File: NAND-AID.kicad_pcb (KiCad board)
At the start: 2 copper layers, 33.7 x 21.4 mm, 20 parts

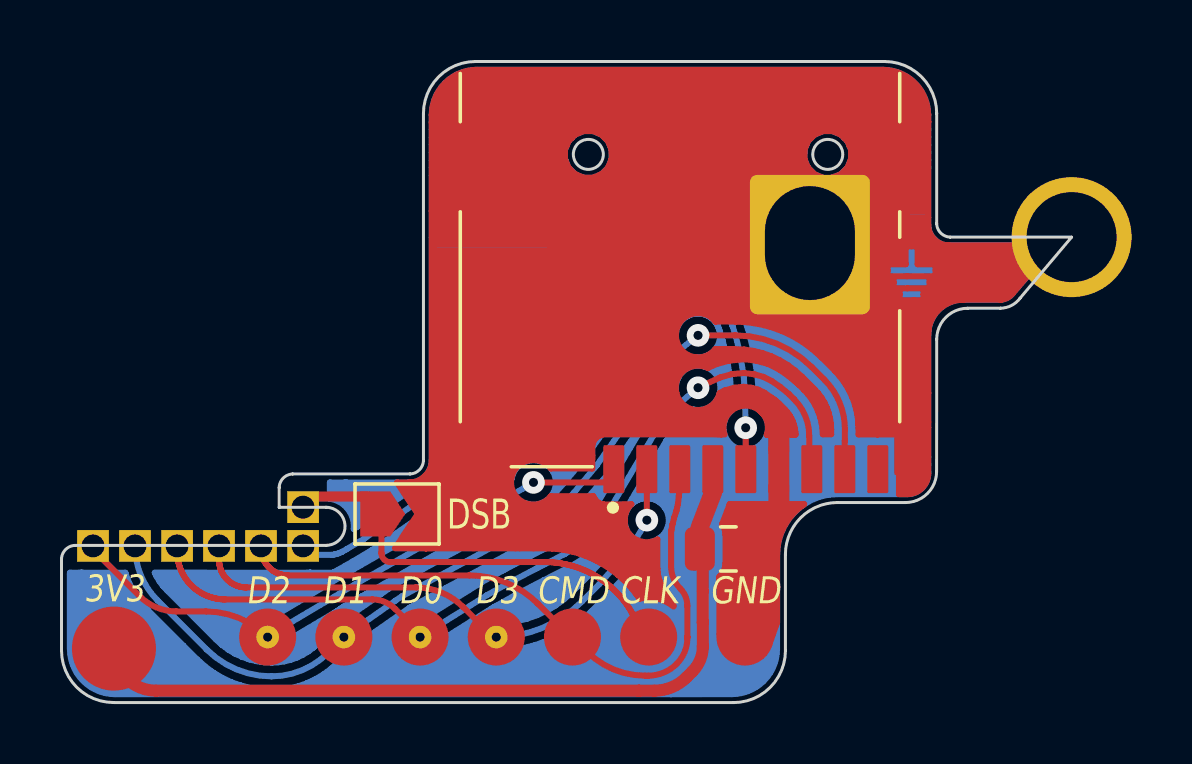
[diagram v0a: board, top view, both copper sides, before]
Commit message: Add logo
Signed-off-by: Thomas Rohloff <v10lator@myway.de>
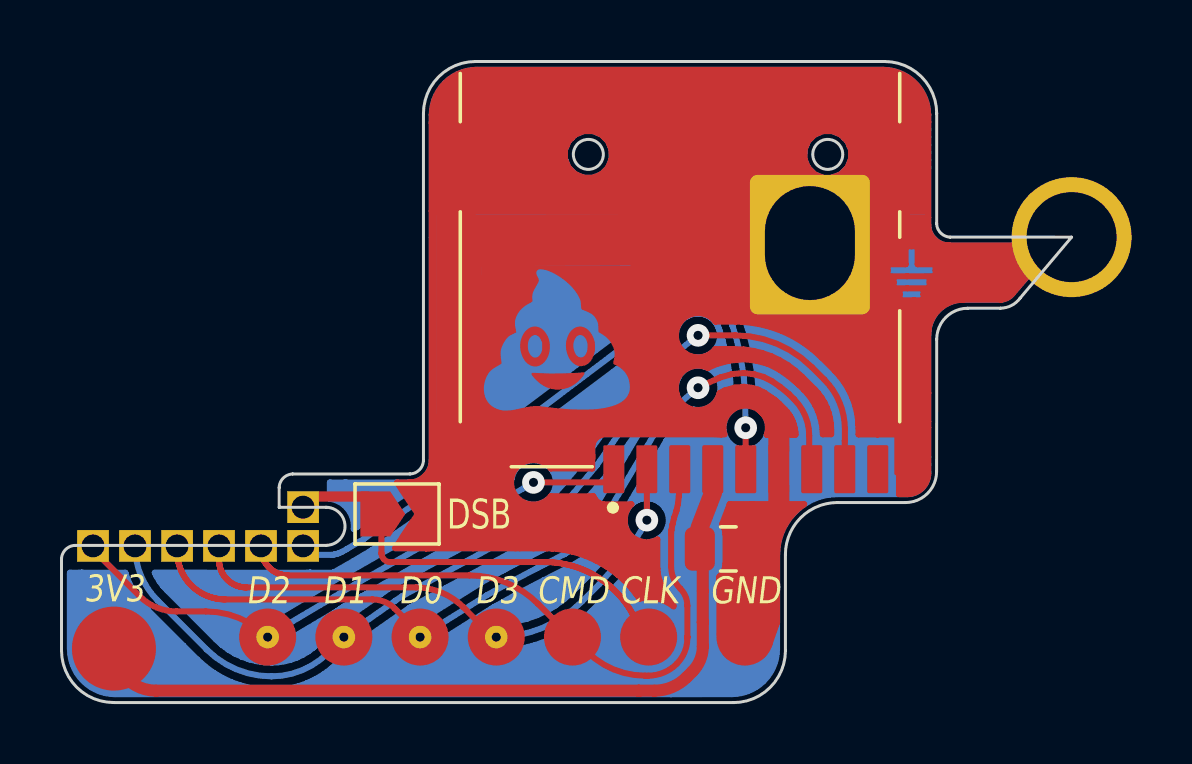
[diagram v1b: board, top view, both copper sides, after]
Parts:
- added G***: LOGO Emoji, V10lator's footprints:LOGO Emoji, F.Cu at (146.0, 99.9)
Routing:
- net GND: track 3466.1 -> 3305.0 mm
